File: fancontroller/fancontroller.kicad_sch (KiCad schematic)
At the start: 24 parts, among them J1 Power, J2 Serial Conn, M1 FAN0, M2 FAN0, M3 FAN0, M4 FAN0, M5 FAN0, M6 FAN0, SW1 SW_Push, U2 ESP32-WROOM-32, U3 AMS1117-3.3

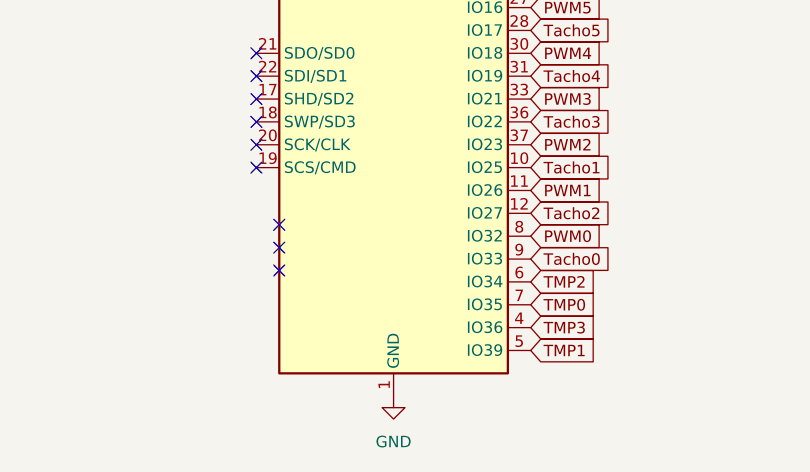
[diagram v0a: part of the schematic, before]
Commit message: First pcb iteration done
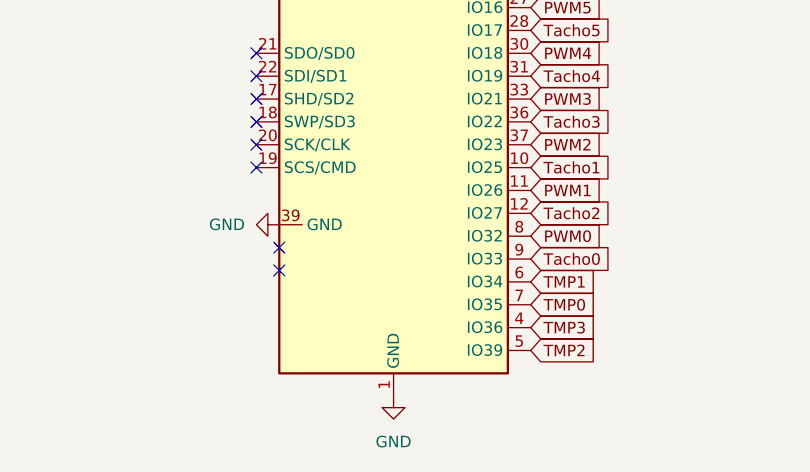
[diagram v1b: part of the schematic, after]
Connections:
- net GND: now also U2.39 (GND)
- net TMP1: now also U2.6 (IO34); no longer U2.5 (SENSOR_VN)
- net TMP2: now also U2.5 (SENSOR_VN); no longer U2.6 (IO34)
- no-connect marks 18 -> 17
